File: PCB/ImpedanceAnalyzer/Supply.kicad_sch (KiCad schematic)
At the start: 52 parts, among them U18 LM7812_TO220, U19 LM7912_TO220, U20 LM7806_TO220, U21 LT1086-3.3, U22 LM7805_TO220, U23 LM7905_TO220, U24 LM7906_TO220

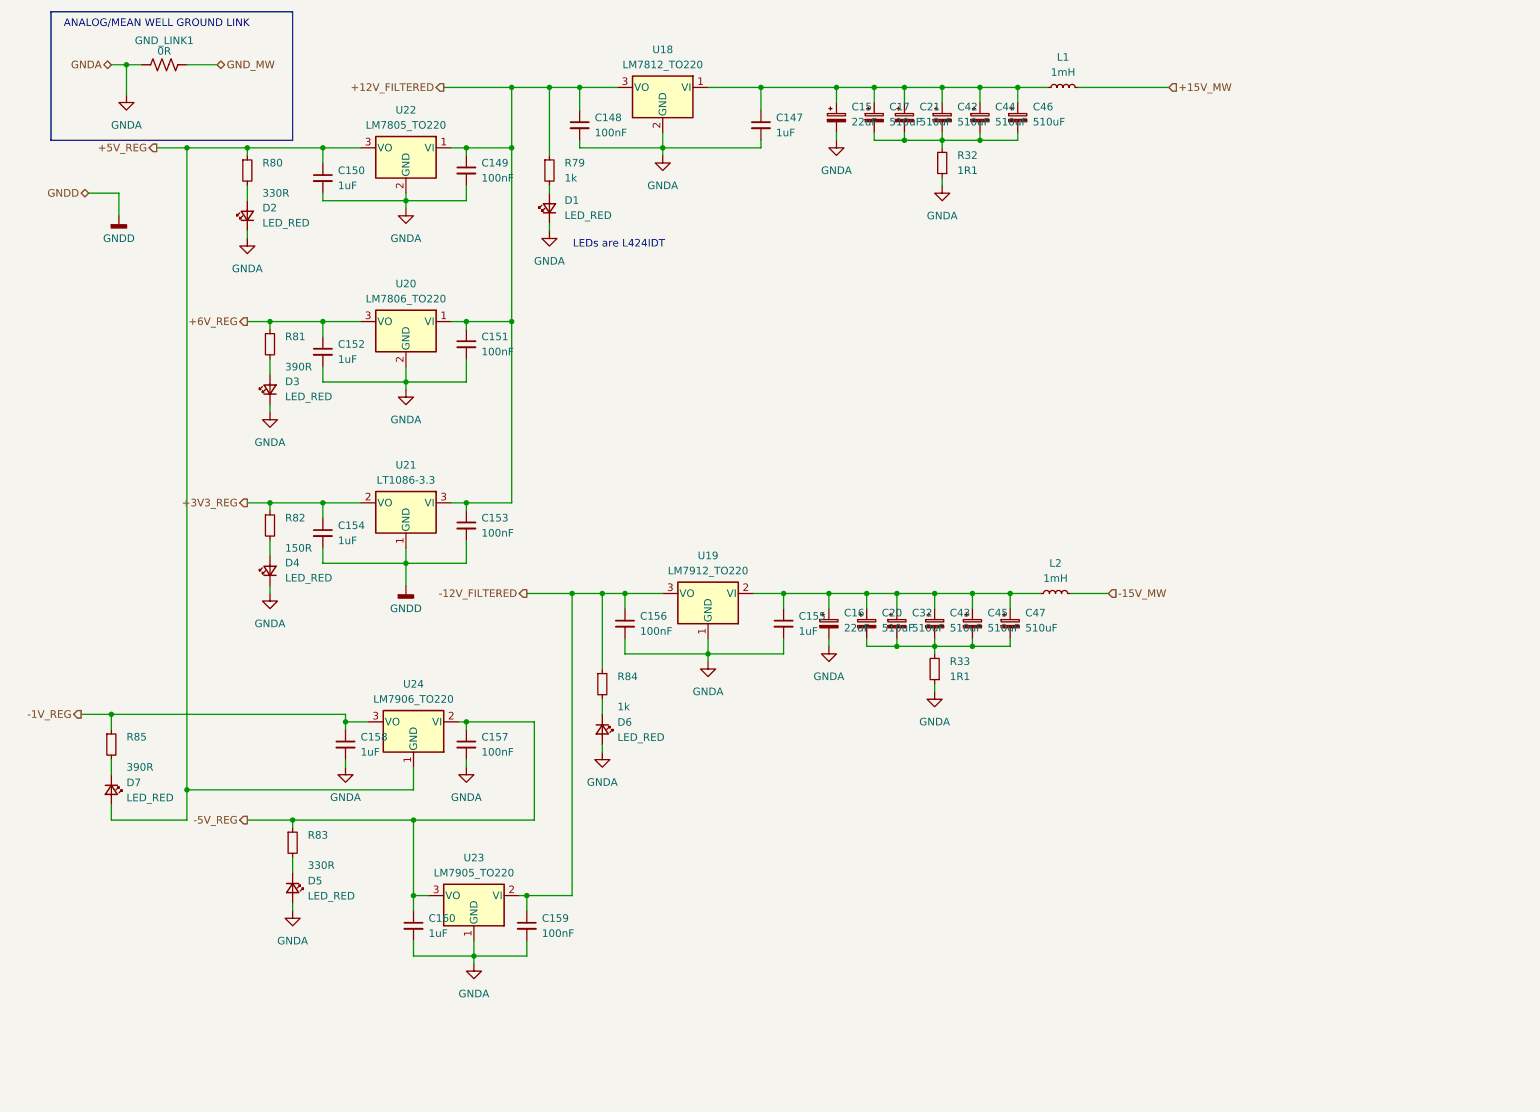
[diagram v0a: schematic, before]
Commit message: corrected kicad
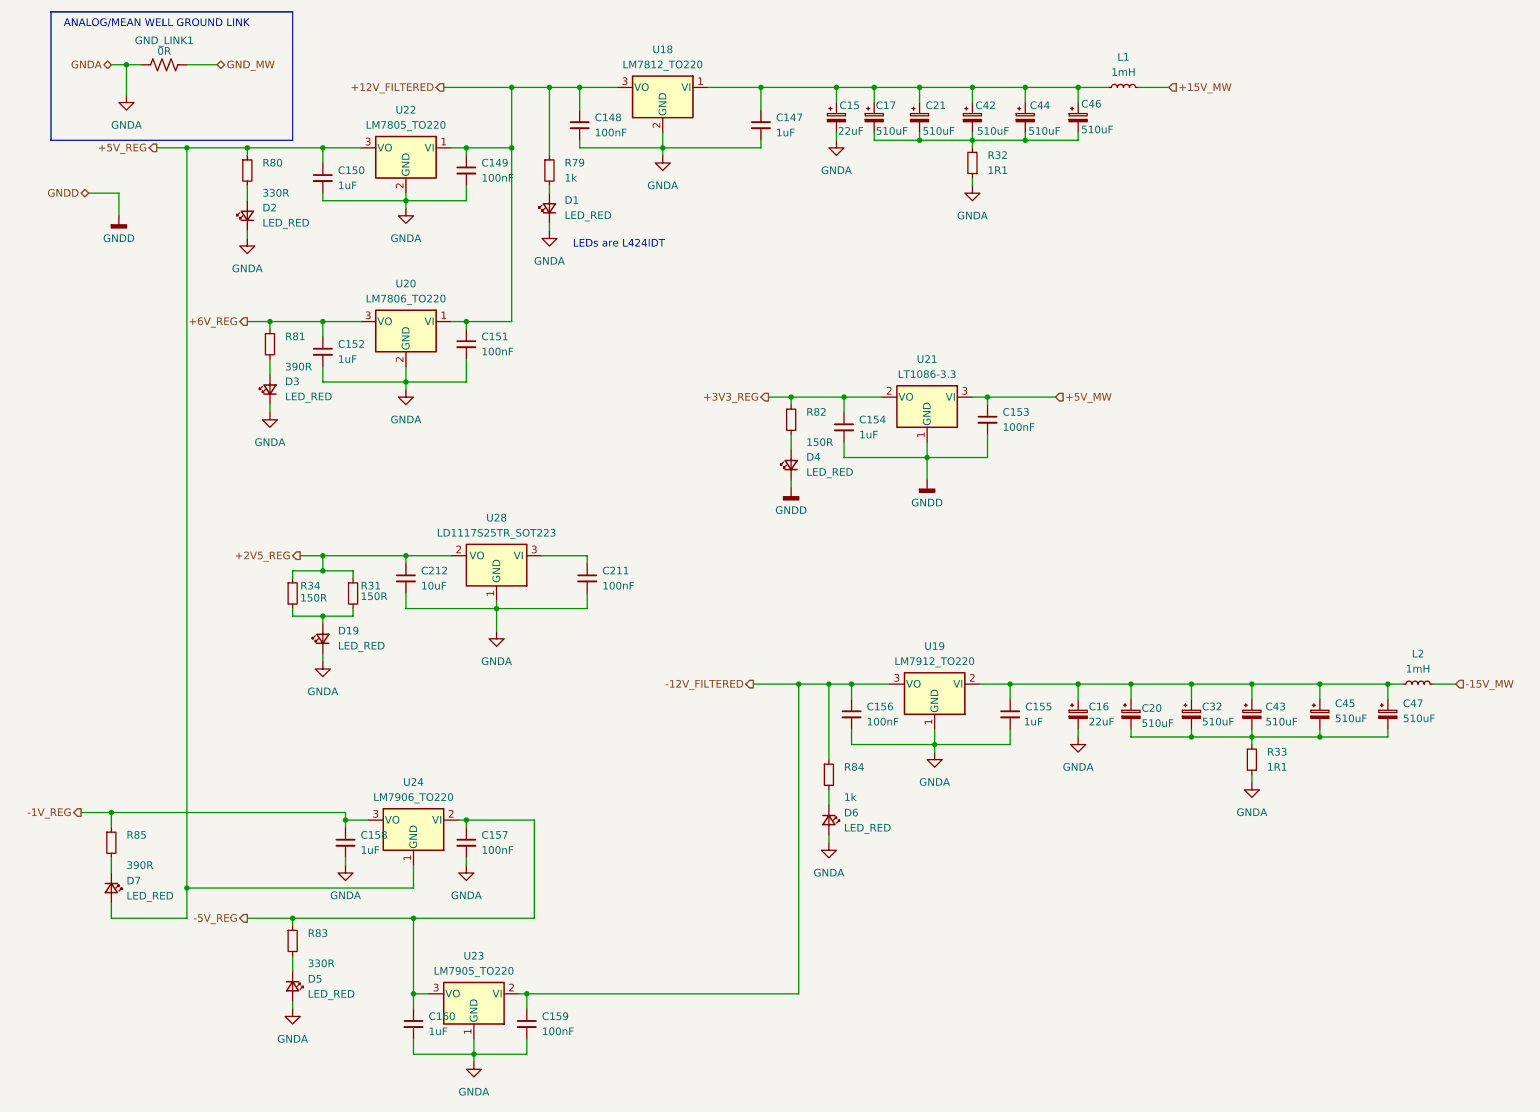
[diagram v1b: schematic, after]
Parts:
- added C211: 100nF, Capacitor_SMD:C_0805_2012Metric_Pad1.18x1.45mm_HandSolder, symbol Device:C_Small
- added C212: 10uF, Capacitor_SMD:C_1210_3225Metric, symbol Device:C_Small
- added D19: LED_RED, LED_THT:LED_D2.0mm_W4.0mm_H2.8mm_FlatTop, symbol Device:LED_Small
- added R31, R34: 150R, Resistor_THT:R_Axial_DIN0207_L6.3mm_D2.5mm_P10.16mm_Horizontal, symbol Device:R_Small
- added U28: LD1117S25TR_SOT223, Package_TO_SOT_SMD:SOT-223-3_TabPin2, symbol Regulator_Linear:LD1117S25TR_SOT223
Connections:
- net +12V_FILTERED: no longer C153.1, U21.3 (VI)
- net GNDA: now also C211.2, C212.2, D19.1 (K), U28.1 (GND); no longer D4.1 (K)
- net GNDD: now also D4.1 (K)
- new net: D19.2 (A), R31.2, R34.2
- new net: C211.1, U28.3 (VI)
- new net +2V5_REG: C212.1, R31.1, R34.1, U28.2 (VO)
- new net +5V_MW: C153.1, U21.3 (VI)
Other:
- moved on the sheet: C153, C154, C155, C156, C157, C158, C159, C16, C160, C20, C21, C32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
